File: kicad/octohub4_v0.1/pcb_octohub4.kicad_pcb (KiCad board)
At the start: 2 copper layers, 100 x 80 mm, 83 parts, among them J101 USB231ARY, J102 USB231ARY, J103 USB231ARY, J104 USB231ARY, J201 Screw_Terminal_01x02, J203 Barrel_Jack_Switch, J301 USB_C_Receptacle_USB2.0, U201 TPS259474LRPWR, U301 AMS1117-3.3, U302 USB2514B_Bi, Y301 24MHz

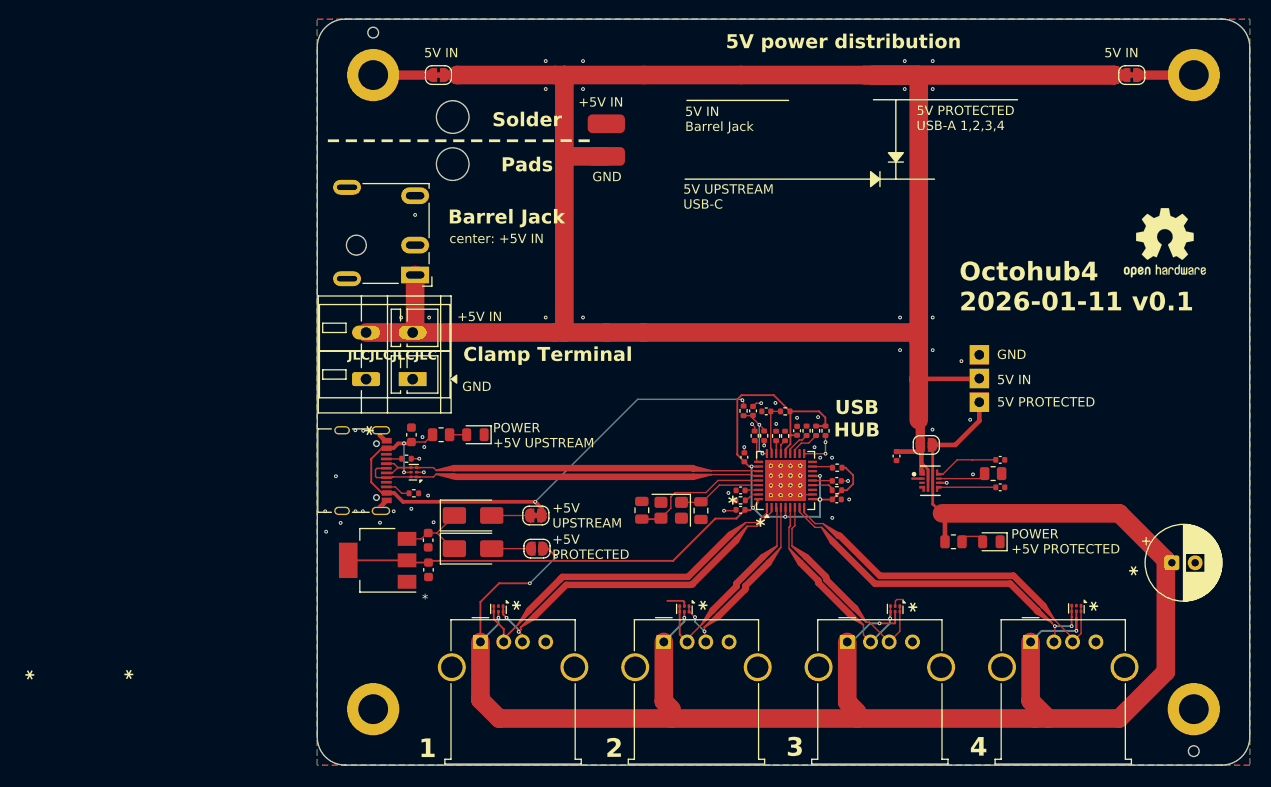
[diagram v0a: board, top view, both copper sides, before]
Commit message: Add run_kicad_purge 4
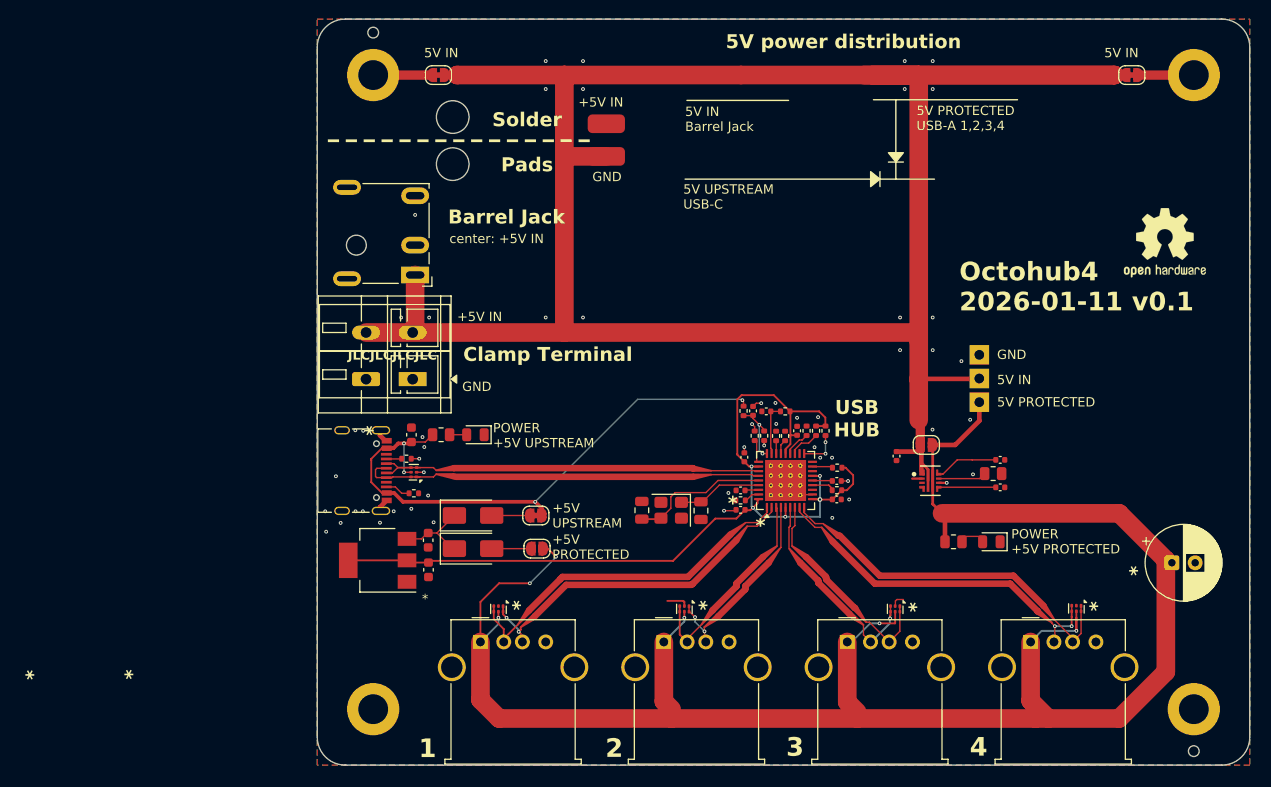
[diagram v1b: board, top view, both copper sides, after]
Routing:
- net Net-(J101-D+): track 5.25 -> 4.56 mm
- net +5VPROTECTED: track 205.7 -> 205.0 mm
- net +3V3: track 99.4 -> 98.8 mm
